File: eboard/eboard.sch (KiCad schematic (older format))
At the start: 81 parts, among them J1 Conn_01x02_Male, J2 USB_B_Micro, J3 Conn_01x03_Male, J4 jst_battery, J5 Conn_01x02_Male, J6 Conn_01x03_Male, Q1 AO4407A_new, Q2 S8050, Q3 S8050, Q6 AO4407A_new, Q7 BSS138K, Q8 BSS138K, SW1 pushbutton_switch, SW2 pushbutton_switch, U1 ESP32-PICO-D4, U2 TPS63000, U3 TP4056, U4 SRV05-4, U5 CP2102, U6 TPS63000

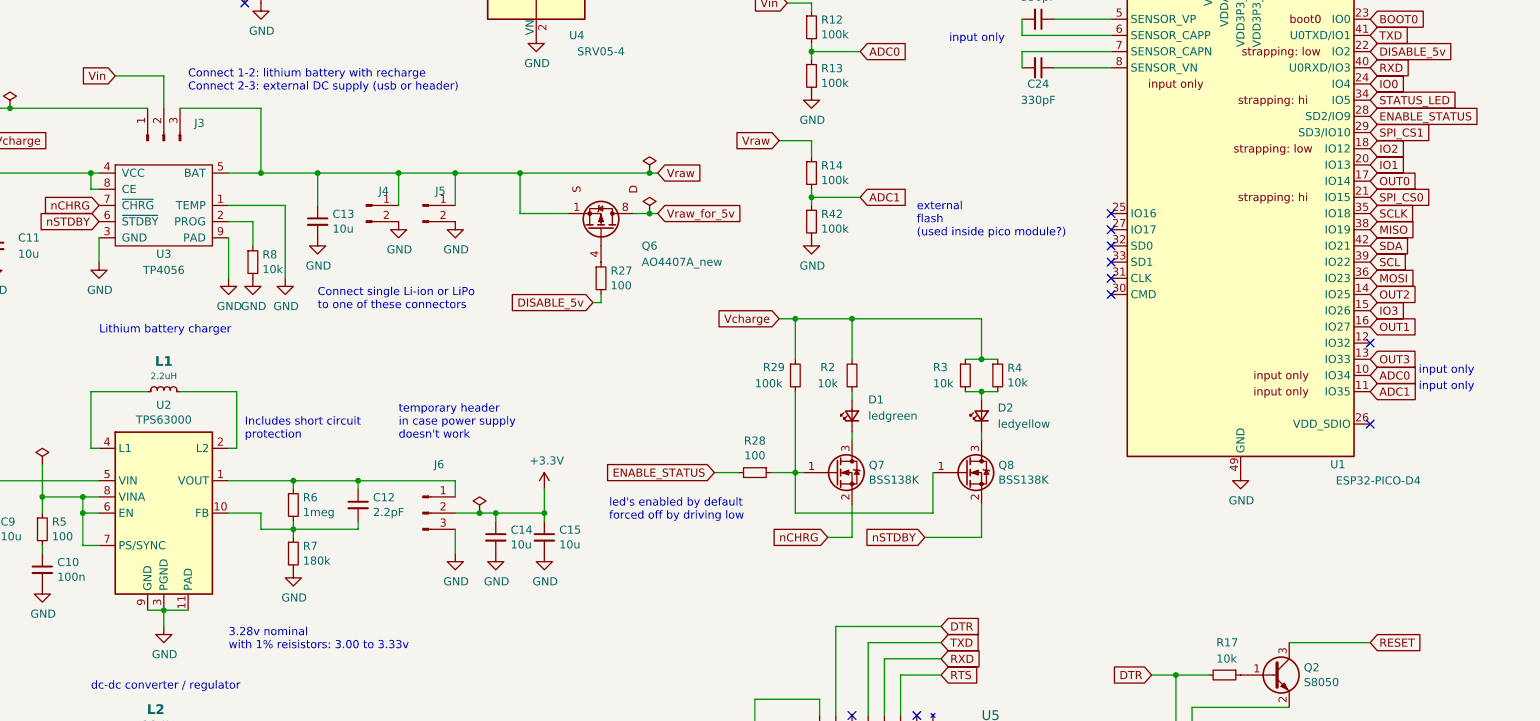
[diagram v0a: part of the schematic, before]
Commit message: routed
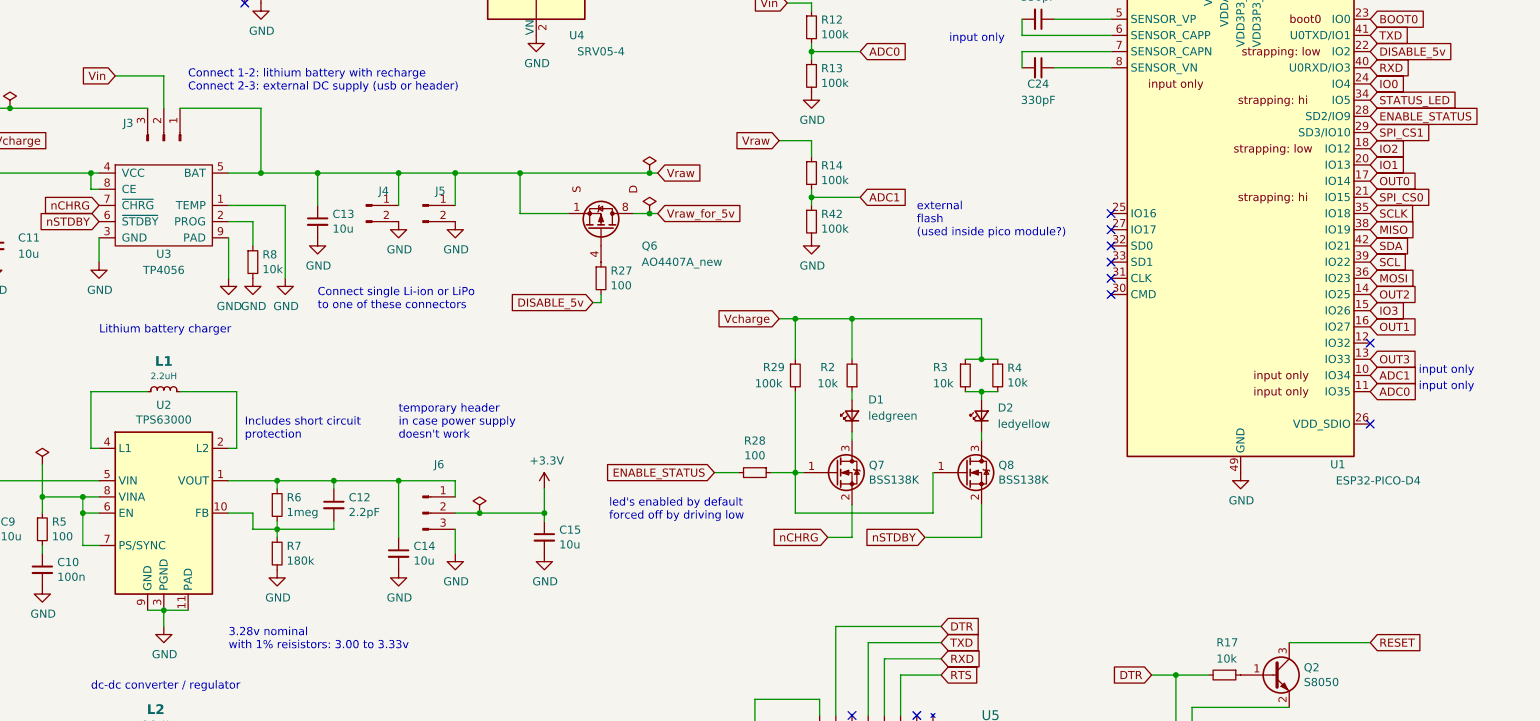
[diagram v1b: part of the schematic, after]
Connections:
- net +3V3: no longer C14.1
- net ADC0: now also U1.11 (IO35); no longer U1.10 (IO34)
- net ADC1: now also U1.10 (IO34); no longer U1.11 (IO35)
- net Vcharge: now also J3.3 (Pin_3); no longer J3.1 (Pin_1)
- net Vraw: now also J3.1 (Pin_1); no longer J3.3 (Pin_3)
- net at C12.1, J6.1 (Pin_1), R6.1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: now also C14.1
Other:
- moved on the sheet: C12, C14, R6, R7
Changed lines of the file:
@@
 F 3 "~" H 2200 2550 50  0001 C CNN
 	1    2200 2550
-	0    -1   -1   0
+	0    1    -1   0
 $EndComp
 Text GLabel 1900 2150 0    50   Input ~ 0
@@
 L pace:1meg R6
 U 1 1 5FA96672
-P 3000 4800
-F 0 "R6" H 3059 4846 50  0000 L CNN
-F 1 "1meg" H 3059 4755 50  0000 L CNN
-F 2 "Resistor_SMD:R_0603_1608Metric" H 3000 4800 50  0001 C CNN
-F 3 "https://lcsc.com/product-detail/Chip-Resistor-Surface-Mount_Uniroyal-Elec-0603WAF1004T5E_C22935.html/?href=jlc-SMT" H 3000 4800 50  0001 C CNN
-F 4 "C22935" H 3000 4800 50  0001 C CNN "LCSC"
-	1    3000 4800
+P 2900 4800
+F 0 "R6" H 2959 4846 50  0000 L CNN
+F 1 "1meg" H 2959 4755 50  0000 L CNN
+F 2 "Resistor_SMD:R_0603_1608Metric" H 2900 4800 50  0001 C CNN
+F 3 "https://lcsc.com/product-detail/Chip-Resistor-Surface-Mount_Uniroyal-Elec-0603WAF1004T5E_C22935.html/?href=jlc-SMT" H 2900 4800 50  0001 C CNN
+F 4 "C22935" H 2900 4800 50  0001 C CNN "LCSC"
+	1    2900 4800
 	1    0    0    -1
 $EndComp
@@
 L pace:180k R7
 U 1 1 5FA97E48
-P 3000 5100
-F 0 "R7" H 3059 5146 50  0000 L CNN
-F 1 "180k" H 3059 5055 50  0000 L CNN
-F 2 "Resistor_SMD:R_0603_1608Metric" H 3000 5100 50  0001 C CNN
-F 3 "https://lcsc.com/product-detail/Chip-Resistor-Surface-Mount_Uniroyal-Elec-0603WAF1803T5E_C22827.html/?href=jlc-SMT" H 3000 5100 50  0001 C CNN
-F 4 "C22827" H 3000 5100 50  0001 C CNN "LCSC"
-	1    3000 5100
-	1    0    0    -1
-$EndComp
-Wire Wire Line
-	2600 4650 3000 4650
-Wire Wire Line
-	3000 4650 3000 4700
-Wire Wire Line
-	3000 4900 3000 4950
+P 2900 5100
+F 0 "R7" H 2959 5146 50  0000 L CNN
+F 1 "180k" H 2959 5055 50  0000 L CNN
+F 2 "Resistor_SMD:R_0603_1608Metric" H 2900 5100 50  0001 C CNN
+F 3 "https://lcsc.com/product-detail/Chip-Resistor-Surface-Mount_Uniroyal-Elec-0603WAF1803T5E_C22827.html/?href=jlc-SMT" H 2900 5100 50  0001 C CNN
+F 4 "C22827" H 2900 5100 50  0001 C CNN "LCSC"
+	1    2900 5100
+	1    0    0    -1
+$EndComp
+Wire Wire Line
+	2600 4650 2900 4650
+Wire Wire Line
+	2900 4650 2900 4700
+Wire Wire Line
+	2900 4900 2900 4950
 $Comp
 L power:GND #PWR?
 U 1 1 5FAA312D
-P 3000 5200
-F 0 "#PWR?" H 3000 4950 50  0001 C CNN
-F 1 "GND" H 3005 5027 50  0000 C CNN
-F 2 "" H 3000 5200 50  0001 C CNN
-F 3 "" H 3000 5200 50  0001 C CNN
-	1    3000 5200
-	1    0    0    -1
-$EndComp
-Wire Wire Line
-	2600 4850 2800 4850
-Wire Wire Line
-	2800 4850 2800 4950
-Wire Wire Line
-	2800 4950 3000 4950
-Connection ~ 3000 4950
-Wire Wire Line
-	3000 4950 3000 5000
+P 2900 5200
+F 0 "#PWR?" H 2900 4950 50  0001 C CNN
+F 1 "GND" H 2905 5027 50  0000 C CNN
+F 2 "" H 2900 5200 50  0001 C CNN
+F 3 "" H 2900 5200 50  0001 C CNN
+	1    2900 5200
+	1    0    0    -1
+$EndComp
+Wire Wire Line
+	2600 4850 2750 4850
+Wire Wire Line
+	2750 4850 2750 4950
+Wire Wire Line
+	2750 4950 2900 4950
+Connection ~ 2900 4950
+Wire Wire Line
+	2900 4950 2900 5000
 Text Notes 2600 5700 0    50   ~ 0
 3.28v nominal\nwith 1% reisistors: 3.00 to 3.33v
@@
 L pace:2.2pF C12
 U 1 1 5FAAD83F
-P 3400 4800
-F 0 "C12" H 3492 4846 50  0000 L CNN
-F 1 "2.2pF" H 3492 4755 50  0000 L CNN
-F 2 "Capacitor_SMD:C_0402_1005Metric" H 3400 4800 50  0001 C CNN
-F 3 "https://lcsc.com/product-detail/Multilayer-Ceramic-Capacitors-MLCC-SMD-SMT_2-2pF-2R2-0-25pF-50V_C1559.html/?href=jlc-SMT" H 3400 4800 50  0001 C CNN
-F 4 "C1559" H 3400 4800 50  0001 C CNN "LCSC"
-	1    3400 4800
-	1    0    0    -1
-$EndComp
-Wire Wire Line
-	3000 4650 3400 4650
-Wire Wire Line
-	3400 4650 3400 4700
-Connection ~ 3000 4650
-Wire Wire Line
-	3000 4950 3400 4950
-Wire Wire Line
-	3400 4950 3400 4900
+P 3250 4800
+F 0 "C12" H 3342 4846 50  0000 L CNN
+F 1 "2.2pF" H 3342 4755 50  0000 L CNN
+F 2 "Capacitor_SMD:C_0402_1005Metric" H 3250 4800 50  0001 C CNN
+F 3 "https://lcsc.com/product-detail/Multilayer-Ceramic-Capacitors-MLCC-SMD-SMT_2-2pF-2R2-0-25pF-50V_C1559.html/?href=jlc-SMT" H 3250 4800 50  0001 C CNN
+F 4 "C1559" H 3250 4800 50  0001 C CNN "LCSC"
+	1    3250 4800
+	1    0    0    -1
+$EndComp
+Wire Wire Line
+	2900 4650 3250 4650
+Wire Wire Line
+	3250 4650 3250 4700
+Connection ~ 2900 4650
+Wire Wire Line
+	2900 4950 3250 4950
+Wire Wire Line
+	3250 4950 3250 4900
 $Comp
 L pace:10u C14
 U 1 1 5FAB3458
-P 4250 5000
-F 0 "C14" H 4342 5046 50  0000 L CNN
-F 1 "10u" H 4342 4955 50  0000 L CNN
-F 2 "Capacitor_SMD:C_0402_1005Metric" H 4250 5000 50  0001 C CNN
-F 3 "https://datasheet.lcsc.com/szlcsc/Samsung-Electro-Mechanics-CL05A106MQ5NUNC_C15525.pdf" H 4250 5000 50  0001 C CNN
-F 4 "C15525" H 4250 5000 50  0001 C CNN "LCSC"
-	1    4250 5000
-	1    0    0    -1
-$EndComp
-Wire Wire Line
-	4250 4850 4250 4900
+P 3650 5100
+F 0 "C14" H 3742 5146 50  0000 L CNN
+F 1 "10u" H 3742 5055 50  0000 L CNN
+F 2 "Capacitor_SMD:C_0402_1005Metric" H 3650 5100 50  0001 C CNN
+F 3 "https://datasheet.lcsc.com/szlcsc/Samsung-Electro-Mechanics-CL05A106MQ5NUNC_C15525.pdf" H 3650 5100 50  0001 C CNN
+F 4 "C15525" H 3650 5100 50  0001 C CNN "LCSC"
+	1    3650 5100
+	1    0    0    -1
+$EndComp
 $Comp
 L power:GND #PWR?
 U 1 1 5FAB6079
-P 4250 5100
-F 0 "#PWR?" H 4250 4850 50  0001 C CNN
-F 1 "GND" H 4255 4927 50  0000 C CNN
-F 2 "" H 4250 5100 50  0001 C CNN
-F 3 "" H 4250 5100 50  0001 C CNN
-	1    4250 5100
+P 3650 5200
+F 0 "#PWR?" H 3650 4950 50  0001 C CNN
+F 1 "GND" H 3655 5027 50  0000 C CNN
+F 2 "" H 3650 5200 50  0001 C CNN
+F 3 "" H 3650 5200 50  0001 C CNN
+	1    3650 5200
 	1    0    0    -1
 $EndComp
@@
 	1    0    0    -1
 $EndComp
-Wire Wire Line
-	4250 4850 4550 4850
 Wire Wire Line
 	4550 4850 4550 4700
@@
 Wire Wire Line
 	4000 4850 4150 4850
-Connection ~ 4250 4850
 Wire Wire Line
 	4000 4750 4000 4650
 Wire Wire Line
-	4000 4650 3400 4650
-Connection ~ 3400 4650
+	4000 4650 3650 4650
+Connection ~ 3250 4650
 Text Notes 3650 4400 0    50   ~ 0
 temporary header\nin case power supply\ndoesn't work\n
@@
 $EndComp
 Connection ~ 4150 4850
-Wire Wire Line
-	4150 4850 4250 4850
 Text GLabel 9650 2500 2    50   Input ~ 0
 SPI_CS1
@@
 Wire Wire Line
 	7500 2000 8050 2000
+Text GLabel 9650 4100 2    50   Input ~ 0
+ADC0
 Text GLabel 9650 4000 2    50   Input ~ 0
-ADC0
-Text GLabel 9650 4100 2    50   Input ~ 0
 ADC1
 $Comp
@@
 Text GLabel 9650 2700 2    50   Input ~ 0
 IO1
+Wire Wire Line
+	4150 4850 4550 4850
+Wire Wire Line
+	3650 5000 3650 4650
+Connection ~ 3650 4650
+Wire Wire Line
+	3650 4650 3250 4650
 $EndSCHEMATC
